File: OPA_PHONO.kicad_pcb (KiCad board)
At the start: 4 copper layers, 99 x 15 mm, 62 parts, among them J1 PJRAS2X1S01X, J2 PJRAS2X1S01X, J3 UJC-HP-3-SMT-TR, U1 OPA1644AxD, U2 OPA1612AxD, U3 LTC3265xDHC

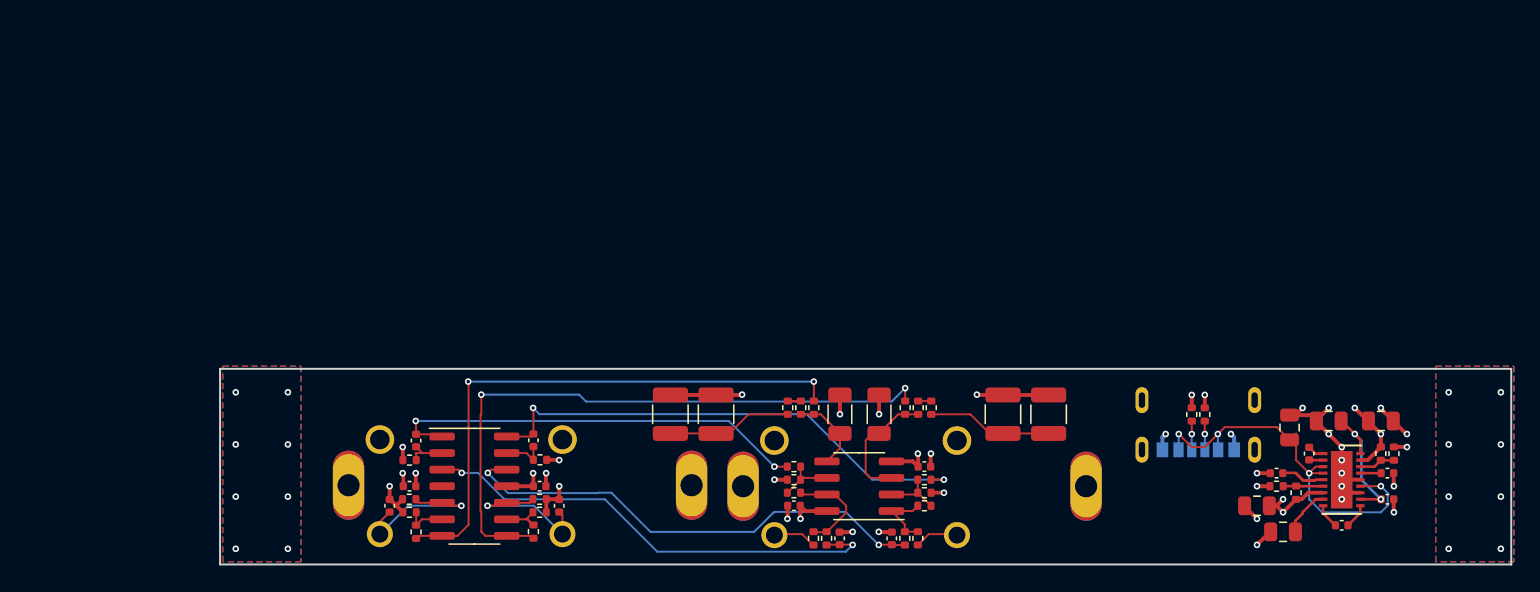
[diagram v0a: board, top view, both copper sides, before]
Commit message: Clean DRC
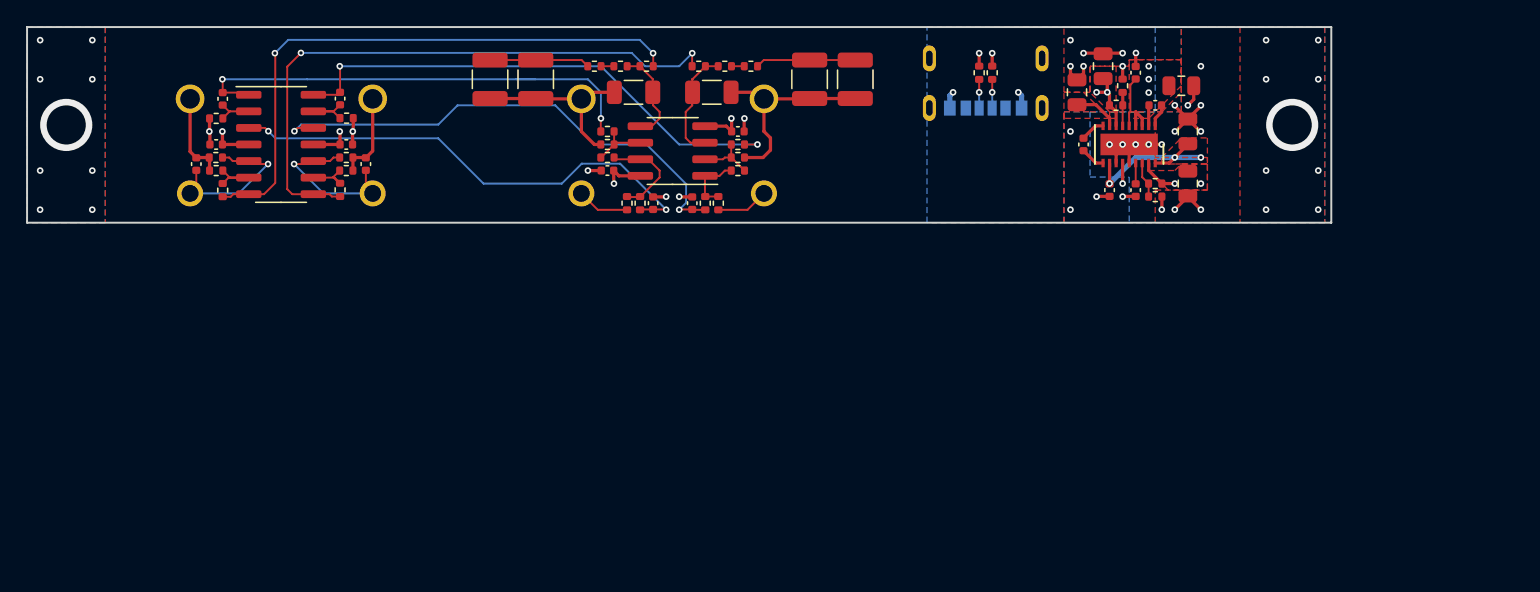
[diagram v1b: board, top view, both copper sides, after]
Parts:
- moved J1 38.0 mm to (153.2, 50.2), turned to 0 degrees
- moved J2 37.9 mm to (123.2, 50.2), turned to 0 degrees
- moved C24 37.2 mm to (180.5, 55.0), turned to -90 degrees
- moved C28 35.7 mm to (182.5, 53.0), turned to 90 degrees
- moved C14 35.3 mm to (181.0, 59.0), turned to -90 degrees
- moved R27 32.9 mm to (184.0, 54.5), turned to -90 degrees
- moved R28 32.8 mm to (183.5, 56.0), turned to 180 degrees
- moved C18 32.5 mm to (185.0, 53.5), turned to 90 degrees
- moved C13 31.9 mm to (183.0, 62.5), turned to 90 degrees
- moved J3 30.9 mm to (173.5, 56.2)
- moved R29 30.9 mm to (174.0, 53.5)
- moved R30 30.9 mm to (173.0, 53.5)
- moved R4 30.6 mm to (151.5, 53.0), turned to 180 degrees
- moved U3 30.4 mm to (184.5, 59.0), turned to -90 degrees
- moved C1 30.1 mm to (126.0, 60.5)
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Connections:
- J3 pad S1: unconnected-(J3-Pad24) -> unconnected-(J3-PadS1)
- J3 pad S2: unconnected-(J3-Pad24) -> unconnected-(J3-PadS2)
- J3 pad S3: unconnected-(J3-Pad24) -> unconnected-(J3-PadS3)
- J3 pad S4: (no net) -> unconnected-(J3-PadS4)
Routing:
- net /POWER/VIN: track 30.1 -> 3.93 mm
- net GND: track 57.2 -> 81.0 mm
- net /LEFT/TRIM: track 33.5 -> 37.0 mm
- net /LEFT/OUT1: track 43.2 -> 45.3 mm
- net /RIGHT/OUT_RC: track 37.1 -> 39.1 mm
- net /RIGHT/RIAA_RC: track 9.61 -> 7.69 mm
- net /LEFT/RIAA_RC: track 9.61 -> 7.69 mm
- net /RIGHT/OUT1: track 48.9 -> 47.0 mm
- net /LEFT/OUT_RC: track 36.3 -> 37.9 mm
- net /POWER/VOUTP: track 11.1 -> 12.5 mm, vias 2 -> 3
- net /POWER/VOUTN: track 4.89 -> 3.52 mm
- net /POWER/BYPN: track 5.03 -> 3.76 mm
- net /RIGHT/FBTRIM: track 3.28 -> 4.51 mm
- net /LEFT/FB1: track 3.18 -> 4.40 mm
- net /OUT_L: track 3.11 -> 4.02 mm
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- added copper zone on F.Cu, net +12V
- added copper zone on F.Cu, net -12V
- added copper zone on B.Cu, net /POWER/VIN
- added copper zone on F.Cu, net /POWER/VIN
- added copper zone on F.Cu, net /POWER/VOUTN
- added copper zone on F.Cu, net /POWER/VOUTP
- removed copper zone on In2.Cu, net GND
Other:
- board size 99 x 15 mm -> 100 x 15 mm
- rule pad_to_mask_clearance: 0 -> 0.0762
